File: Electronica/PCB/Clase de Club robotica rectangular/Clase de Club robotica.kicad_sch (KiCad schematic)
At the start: 17 parts, among them J1 Ultrasonico 1, J2 Screw_Terminal_01x02, J3 Ultrasonico 2, J4 Ultrasonico 3, J6 Screw_Terminal_01x02, SW1 SW_SPST, SW2 SW_Push

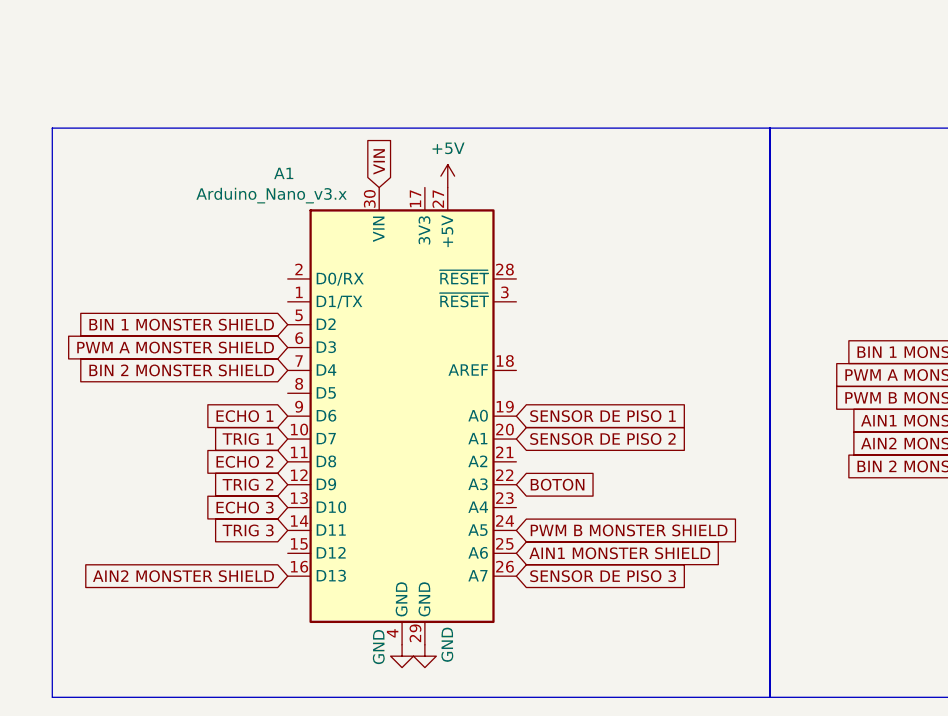
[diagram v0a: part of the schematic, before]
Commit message: Me quiero cortar las bolas
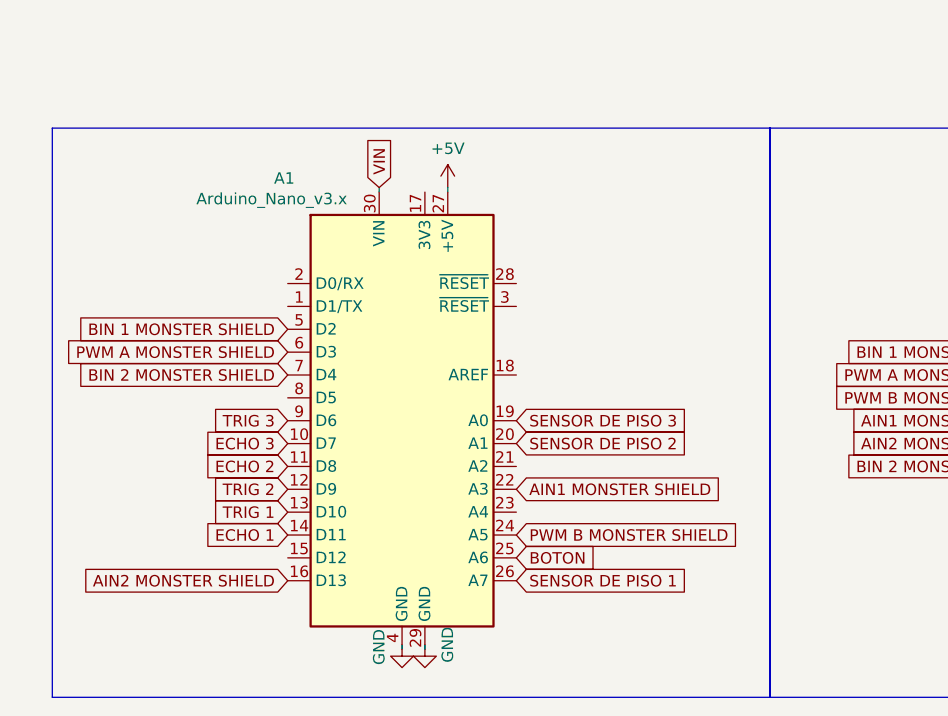
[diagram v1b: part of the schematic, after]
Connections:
- net AIN1 MONSTER SHIELD: now also A1.22 (A3); no longer A1.25 (A6)
- net BOTON : now also A1.25 (A6); no longer A1.22 (A3)
- net ECHO 1: now also A1.14 (D11); no longer A1.9 (D6)
- net ECHO 3: now also A1.10 (D7); no longer A1.13 (D10)
- net SENSOR DE PISO 1: now also A1.26 (A7); no longer A1.19 (A0)
- net SENSOR DE PISO 3: now also A1.19 (A0); no longer A1.26 (A7)
- net TRIG 1: now also A1.13 (D10); no longer A1.10 (D7)
- net TRIG 3: now also A1.9 (D6); no longer A1.14 (D11)
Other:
- moved on the sheet: A1
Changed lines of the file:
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@@
 	(wire
 		(pts
+			(xy 50.8 69.85) (xy 50.8 69.342)
+		)
+		(stroke
+			(width 0)
+			(type default)
+		)
+	)
+	(wire
+		(pts
 			(xy 238.252 66.548) (xy 237.49 66.548)
 		)
@@
 	(wire
 		(pts
+			(xy 55.88 19.05) (xy 55.88 18.542)
+		)
+		(stroke
+			(width 0)
+			(type default)
+		)
+	)
+	(wire
+		(pts
 			(xy 233.934 20.828) (xy 244.094 20.828)
 		)
@@
 	(wire
 		(pts
+			(xy 53.34 69.85) (xy 53.34 69.342)
+		)
+		(stroke
+			(width 0)
+			(type default)
+		)
+	)
+	(wire
+		(pts
 			(xy 215.138 54.61) (xy 219.964 54.61)
 		)
@@
 		)
 	)
+	(wire
+		(pts
+			(xy 48.26 19.05) (xy 48.26 18.542)
+		)
+		(stroke
+			(width 0)
+			(type default)
+		)
+	)
 	(rectangle
 		(start 200.152 45.974)
@@
 	(global_label "TRIG 3"
 		(shape input)
-		(at 38.1 56.642 180)
+		(at 38.1 44.45 180)
 		(fields_autoplaced yes)
 		(effects
@@
 		)
 		(property "Intersheetrefs" "${INTERSHEET_REFS}"
-			(at 28.8253 56.642 0)
+			(at 28.8253 44.45 0)
 			(effects
 				(font
@@
 		)
 	)
+	(global_label "AIN1 MONSTER SHIELD"
+		(shape input)
+		(at 63.5 52.07 0)
+		(fields_autoplaced yes)
+		(effects
+			(font
+				(size 1.27 1.27)
+			)
+			(justify left)
+		)
+		(property "Intersheetrefs" "${INTERSHEET_REFS}"
+			(at 87.9542 52.07 0)
+			(effects
+				(font
+					(size 1.27 1.27)
+				)
+				(justify left)
+				(hide yes)
+			)
+		)
+	)
 	(global_label "BIN 1 MONSTER SHIELD"
 		(shape input)
@@
 	(global_label "BIN 2 MONSTER SHIELD"
 		(shape input)
-		(at 38.1 38.862 180)
+		(at 38.1 39.37 180)
 		(fields_autoplaced yes)
 		(effects
@@
 		)
 		(property "Intersheetrefs" "${INTERSHEET_REFS}"
-			(at 12.4968 38.862 0)
+			(at 12.4968 39.37 0)
 			(effects
 				(font
@@
 	(global_label "ECHO 2"
 		(shape input)
-		(at 38.1 49.022 180)
+		(at 38.1 49.53 180)
 		(fields_autoplaced yes)
 		(effects
@@
 		)
 		(property "Intersheetrefs" "${INTERSHEET_REFS}"
-			(at 27.8577 49.022 0)
+			(at 27.8577 49.53 0)
 			(effects
 				(font
@@
 	(global_label "SENSOR DE PISO 2"
 		(shape input)
-		(at 63.5 46.482 0)
+		(at 63.5 46.99 0)
 		(fields_autoplaced yes)
 		(effects
@@
 		)
 		(property "Intersheetrefs" "${INTERSHEET_REFS}"
-			(at 84.9303 46.482 0)
+			(at 84.9303 46.99 0)
 			(effects
 				(font
@@
 	(global_label "ECHO 1"
 		(shape input)
-		(at 38.1 43.942 180)
+		(at 38.1 57.15 180)
 		(fields_autoplaced yes)
 		(effects
@@
 		)
 		(property "Intersheetrefs" "${INTERSHEET_REFS}"
-			(at 27.8577 43.942 0)
+			(at 27.8577 57.15 0)
 			(effects
 				(font
@@
 		)
 	)
-	(global_label "AIN1 MONSTER SHIELD"
-		(shape input)
-		(at 63.5 59.182 0)
-		(fields_autoplaced yes)
-		(effects
-			(font
-				(size 1.27 1.27)
-			)
-			(justify left)
-		)
-		(property "Intersheetrefs" "${INTERSHEET_REFS}"
-			(at 87.9542 59.182 0)
-			(effects
-				(font
-					(size 1.27 1.27)
-				)
-				(justify left)
-				(hide yes)
-			)
-		)
-	)
 	(global_label "ECHO 2"
 		(shape input)
@@
 	(global_label "TRIG 2"
 		(shape input)
-		(at 38.1 51.562 180)
+		(at 38.1 52.07 180)
 		(fields_autoplaced yes)
 		(effects
@@
 		)
 		(property "Intersheetrefs" "${INTERSHEET_REFS}"
-			(at 28.8253 51.562 0)
+			(at 28.8253 52.07 0)
 			(effects
 				(font
@@
 	(global_label "TRIG 1"
 		(shape input)
-		(at 38.1 46.482 180)
+		(at 38.1 54.61 180)
 		(fields_autoplaced yes)
 		(effects
@@
 		)
 		(property "Intersheetrefs" "${INTERSHEET_REFS}"
-			(at 28.8253 46.482 0)
+			(at 28.8253 54.61 0)
 			(effects
 				(font
@@
 	(global_label "BOTON "
 		(shape input)
-		(at 63.5 51.562 0)
+		(at 63.5 59.69 0)
 		(fields_autoplaced yes)
 		(effects
@@
 		)
 		(property "Intersheetrefs" "${INTERSHEET_REFS}"
-			(at 73.6819 51.562 0)
+			(at 73.6819 59.69 0)
 			(effects
 				(font
@@
 	(global_label "PWM B MONSTER SHIELD"
 		(shape input)
-		(at 63.5 56.642 0)
+		(at 63.5 57.15 0)
 		(fields_autoplaced yes)
 		(effects
@@
 		)
 		(property "Intersheetrefs" "${INTERSHEET_REFS}"
-			(at 90.1312 56.642 0)
+			(at 90.1312 57.15 0)
 			(effects
 				(font
@@
 	(global_label "SENSOR DE PISO 1"
 		(shape input)
-		(at 63.5 43.942 0)
+		(at 63.5 62.23 0)
 		(fields_autoplaced yes)
 		(effects
@@
 		)
 		(property "Intersheetrefs" "${INTERSHEET_REFS}"
-			(at 84.9303 43.942 0)
+			(at 84.9303 62.23 0)
 			(effects
 				(font
@@
 	(global_label "BIN 1 MONSTER SHIELD"
 		(shape input)
-		(at 38.1 33.782 180)
+		(at 38.1 34.29 180)
 		(fields_autoplaced yes)
 		(effects
@@
 		)
 		(property "Intersheetrefs" "${INTERSHEET_REFS}"
-			(at 12.4968 33.782 0)
+			(at 12.4968 34.29 0)
 			(effects
 				(font
@@
 	(global_label "PWM A MONSTER SHIELD"
 		(shape input)
-		(at 38.1 36.322 180)
+		(at 38.1 36.83 180)
 		(fields_autoplaced yes)
 		(effects
@@
 		)
 		(property "Intersheetrefs" "${INTERSHEET_REFS}"
-			(at 11.6502 36.322 0)
+			(at 11.6502 36.83 0)
 			(effects
 				(font
@@
 	(global_label "AIN2 MONSTER SHIELD"
 		(shape input)
-		(at 38.1 61.722 180)
+		(at 38.1 62.23 180)
 		(fields_autoplaced yes)
 		(effects
@@
 		)
 		(property "Intersheetrefs" "${INTERSHEET_REFS}"
-			(at 13.6458 61.722 0)
+			(at 13.6458 62.23 0)
 			(effects
 				(font
@@
 	(global_label "SENSOR DE PISO 3"
 		(shape input)
-		(at 63.5 61.722 0)
+		(at 63.5 44.45 0)
 		(fields_autoplaced yes)
 		(effects
@@
 		)
 		(property "Intersheetrefs" "${INTERSHEET_REFS}"
-			(at 84.9303 61.722 0)
+			(at 84.9303 44.45 0)
 			(effects
 				(font
@@
 	(global_label "ECHO 3"
 		(shape input)
-		(at 38.1 54.102 180)
+		(at 38.1 46.99 180)
 		(fields_autoplaced yes)
 		(effects
@@
 		)
 		(property "Intersheetrefs" "${INTERSHEET_REFS}"
-			(at 27.8577 54.102 0)
+			(at 27.8577 46.99 0)
 			(effects
 				(font
@@
 	(symbol
 		(lib_id "MCU_Module:Arduino_Nano_v3.x")
-		(at 50.8 43.942 0)
+		(at 50.8 44.45 0)
 		(unit 1)
 		(exclude_from_sim no)
@@
 		(dnp no)
 		(property "Reference" "A1"
-			(at 36.576 17.018 0)
+			(at 36.576 17.526 0)
 			(effects
 				(font
@@
 		)
 		(property "Value" "Arduino_Nano_v3.x"
-			(at 27.94 19.304 0)
+			(at 27.94 19.812 0)
 			(effects
 				(font
@@
 		)
 		(property "Footprint" "Module:Arduino_Nano"
-			(at 50.8 43.942 0)
+			(at 50.8 44.45 0)
 			(effects
 				(font
@@
 		)
 		(property "Datasheet" "http://www.mouser.com/pdfdocs/Gravitech_Arduino_Nano3_0.pdf"
-			(at 50.8 43.942 0)
+			(at 50.8 44.45 0)
 			(effects
 				(font
@@
 		)
 		(property "Description" "Arduino Nano v3.x"
-			(at 50.8 43.942 0)
+			(at 50.8 44.45 0)
 			(effects
 				(font
